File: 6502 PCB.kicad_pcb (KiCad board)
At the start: 2 copper layers, 23 parts, among them J1 power_source, SW1 RESET, SW2 SW_Push, SW3 SW_Push, SW4 SW_Push, SW5 SW_Push, SW6 SW_Push, U1 W65C02S, U2 28C256, U3 62256, U4 W65C22, U5 74HC00, X1 1MHz

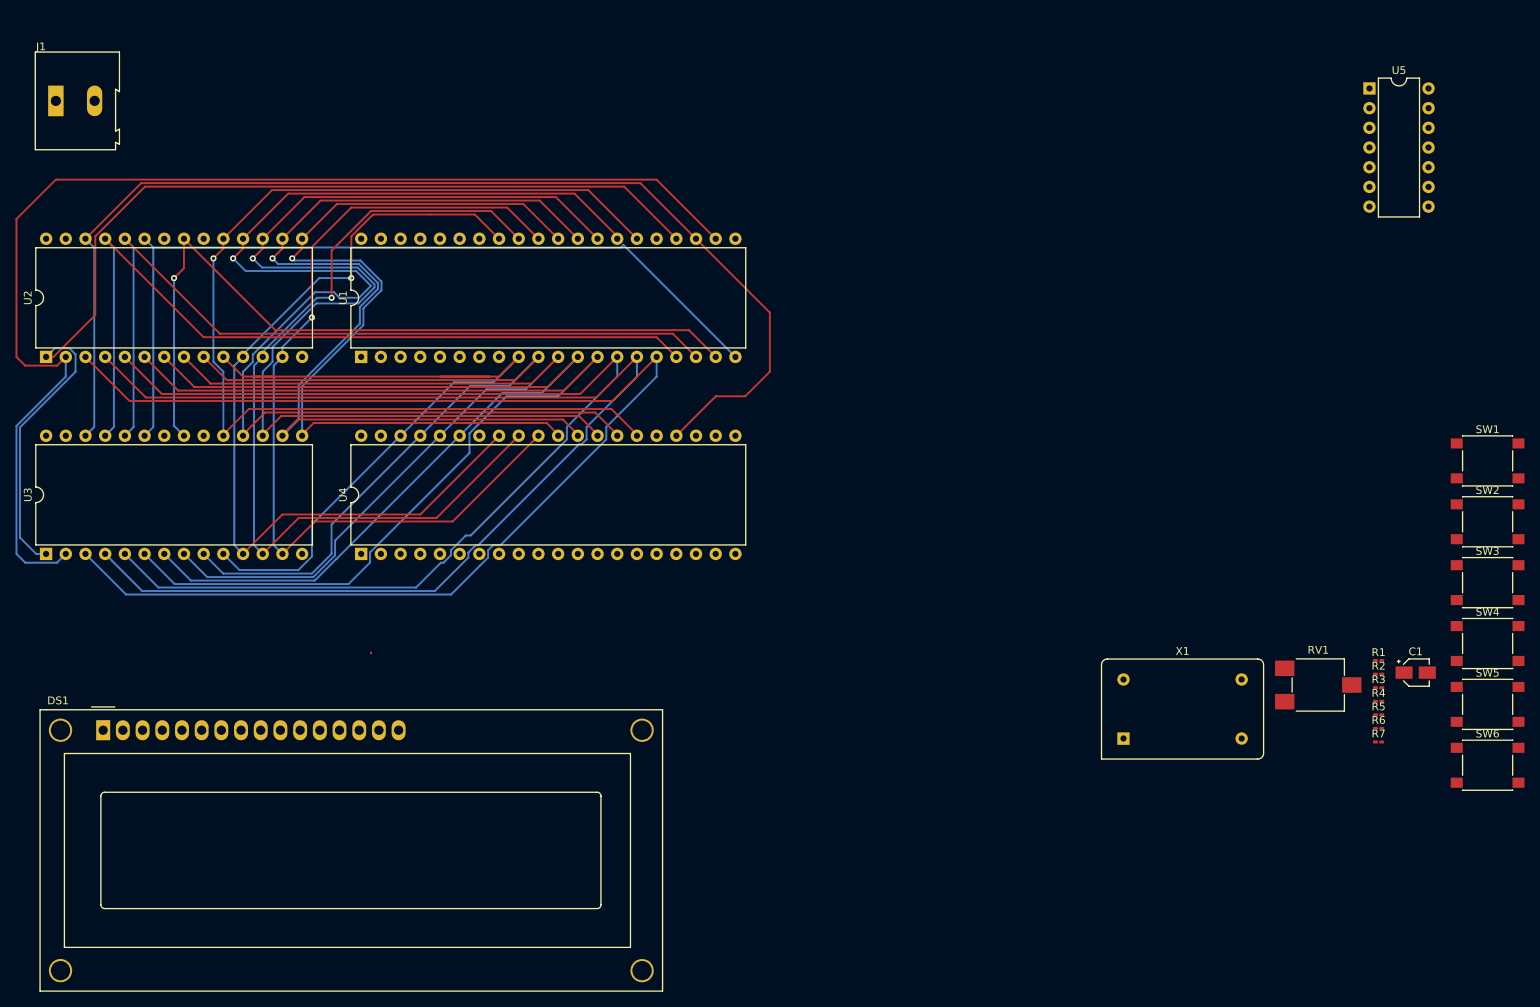
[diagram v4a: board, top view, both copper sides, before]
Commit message: Add files via upload
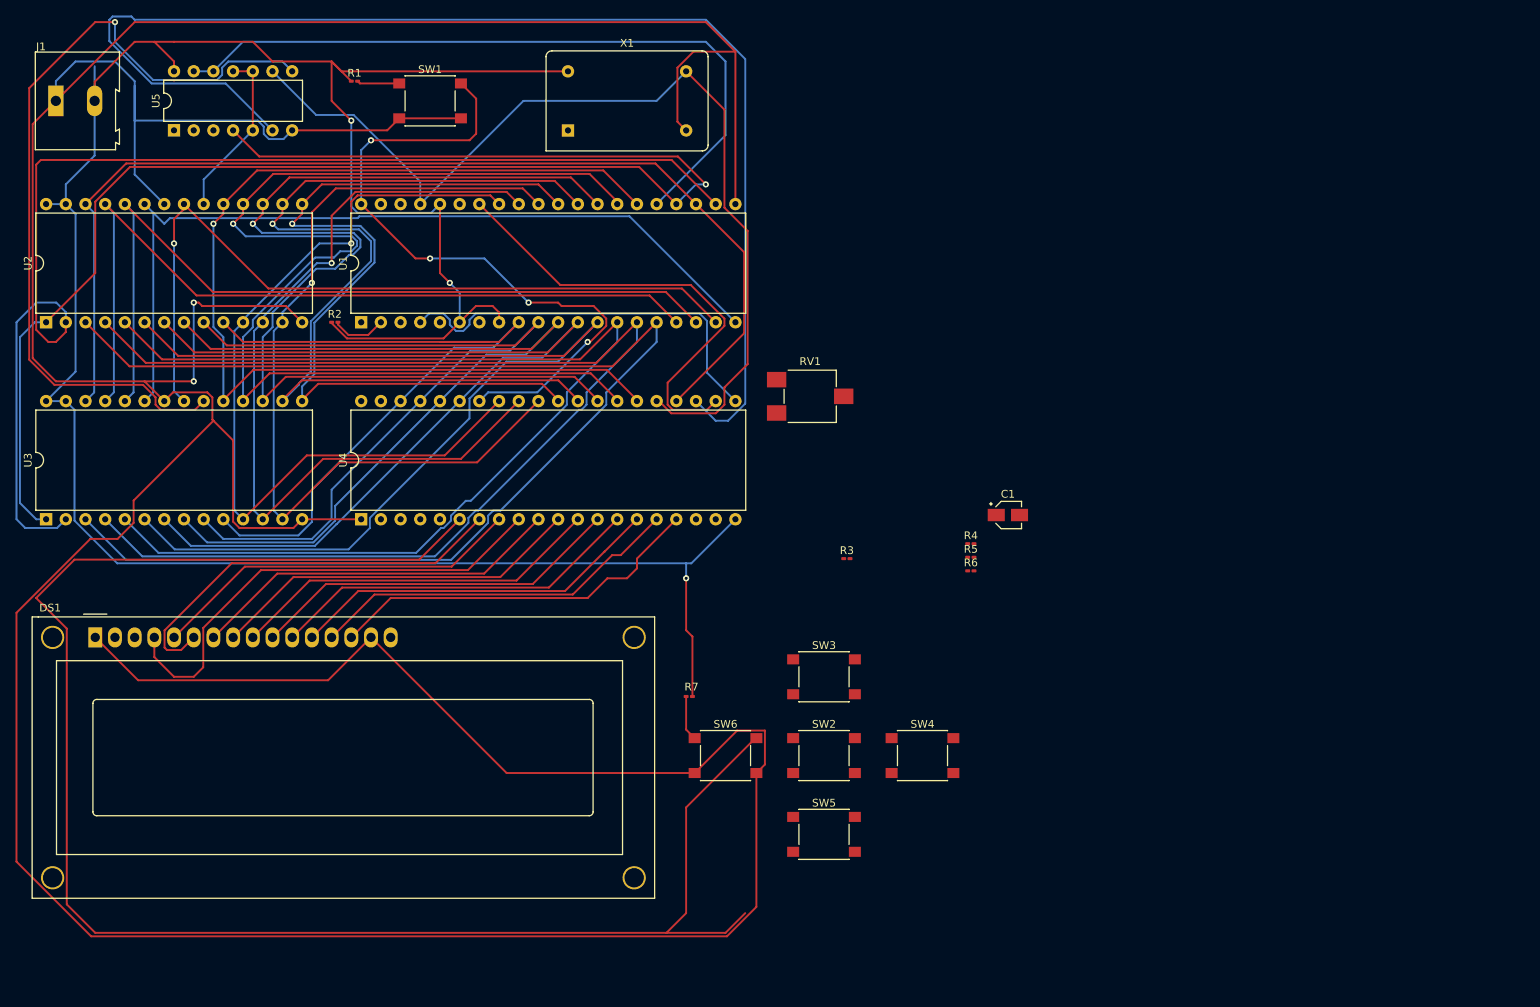
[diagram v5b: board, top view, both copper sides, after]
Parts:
- moved U5 154.3 mm to (33.0, 26.7), turned to 90 degrees
- moved R1 151.7 mm to (56.3, 20.3)
- moved SW1 144.1 mm to (66.0, 22.9)
- moved R2 142.1 mm to (53.7, 51.4)
- moved X1 106.2 mm to (83.8, 26.7)
- moved SW6 98.3 mm to (104.1, 107.3)
- moved SW2 90.7 mm to (116.8, 107.3)
- moved R7 89.1 mm to (99.5, 99.7)
- moved SW5 87.2 mm to (116.8, 117.5)
- moved SW3 86.4 mm to (116.8, 97.1)
- moved RV1 75.4 mm to (115.1, 61.0)
- moved SW4 74.3 mm to (129.5, 107.3)
- moved R3 70.6 mm to (119.8, 81.9)
- moved R4 56.4 mm to (135.8, 80.0)
- moved R5 56.4 mm to (135.8, 81.7)
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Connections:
- U5 pad 14: (no net) -> /VDD
- U5 pad 7: (no net) -> /GND
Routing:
- net /GND: track 0.15 -> 632.1 mm, vias 0 -> 2
- net /VDD: track 0.00 -> 325.0 mm, vias 0 -> 3
- net Net-(U4-PA4): track 0.00 -> 225.8 mm
- net Net-(U4-~{CS2}): track 0.00 -> 165.8 mm
- net Net-(U1-ϕ0): track 0.00 -> 127.0 mm
- net Net-(U3-~{CS}): track 0.00 -> 105.3 mm, vias 0 -> 1
- net Net-(U1-~{RES}): track 0.00 -> 94.5 mm, vias 0 -> 4
- net /a15: track 0.00 -> 93.3 mm
- net Net-(DS1-RS): track 0.00 -> 62.0 mm
- net /a14: track 134.6 -> 195.5 mm, vias 0 -> 1
- net Net-(U1-R/~{W}): track 0.00 -> 58.8 mm
- net Net-(DS1-E): track 0.00 -> 53.3 mm
- net Net-(U1-~{IRQ}): track 0.00 -> 52.3 mm
- net Net-(DS1-D7): track 0.00 -> 49.0 mm
- net Net-(DS1-D3): track 0.00 -> 48.2 mm
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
